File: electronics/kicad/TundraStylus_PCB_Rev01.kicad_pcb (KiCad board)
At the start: 2 copper layers, 80 x 16 mm, 11 parts, among them J1 CON_TPAD, J2 CON_MENU, J3 CON_TRIG, J4 CON_GRIP, SW1 TPAD, SW2 MENU, SW3 TRIG, SW4 GRIP

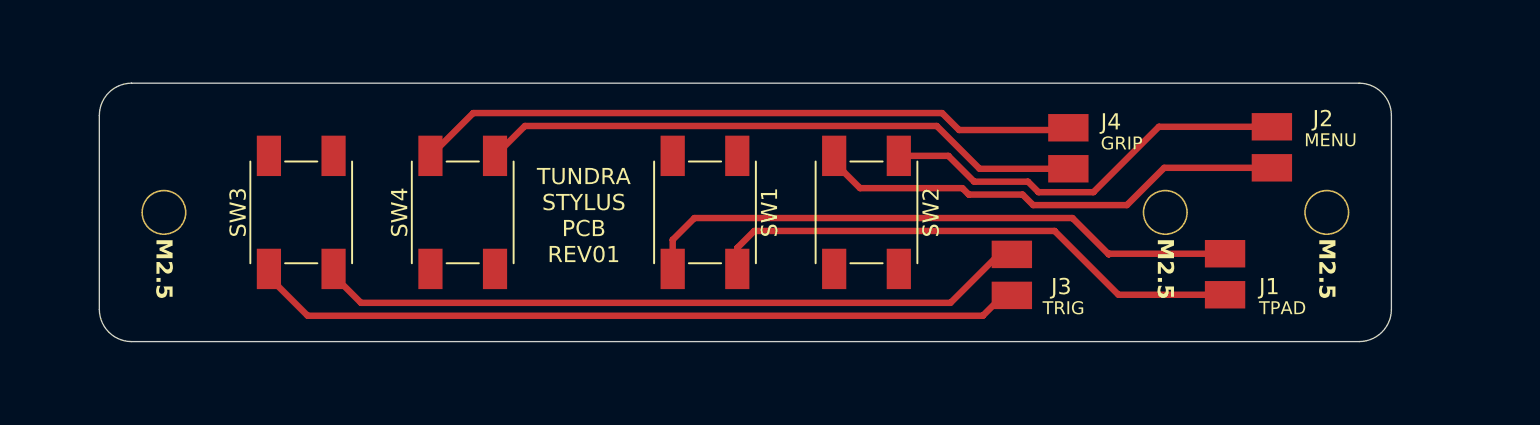
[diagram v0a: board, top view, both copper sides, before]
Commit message: Add latest electronics design
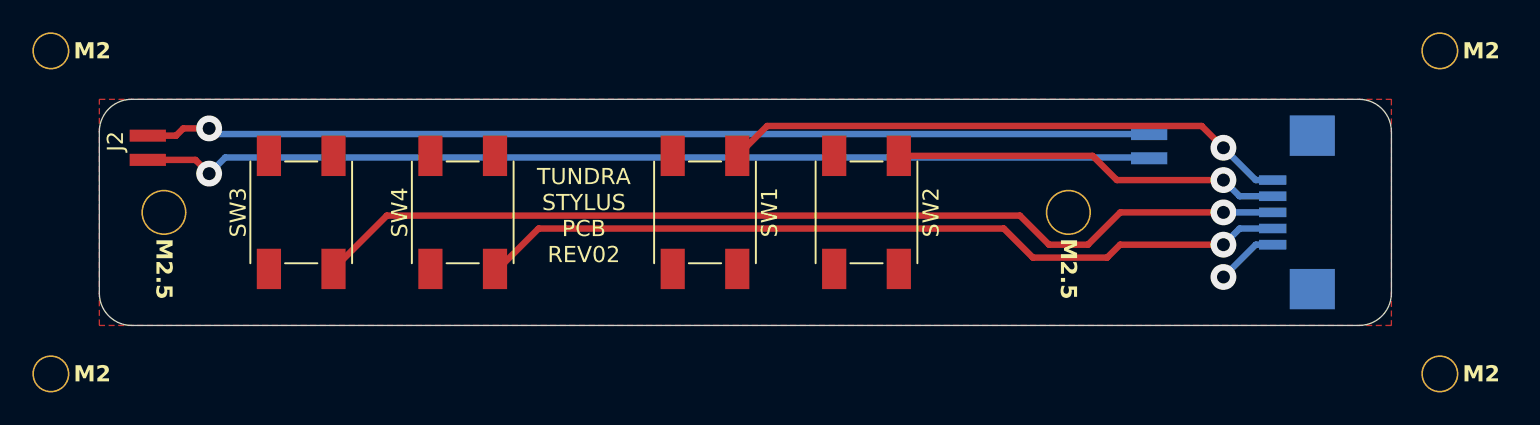
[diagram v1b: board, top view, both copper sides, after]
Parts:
- removed J3: CON_TRIG, fab:PinHeader_1x02_P2.54mm_Horizontal_SMD
- removed J4: CON_GRIP, fab:PinHeader_1x02_P2.54mm_Horizontal_SMD
- added H4: ~, fab:MountingHole_M2, F.Cu at (92.0, 108.0)
- added H5: ~, fab:MountingHole_M2, F.Cu at (178.0, 88.0)
- added H6: ~, fab:MountingHole_M2, F.Cu at (178.0, 108.0)
- added P1: IO, TundraIO:Conn_FFC_1x05_P1mm_SideEntry_GCT_FFC3B11-05-T, B.Cu at (168.7, 98.0)
- H2: footprint fab:MountingHole_M2.5 -> fab:MountingHole_M2
- J1: value CON_TPAD -> HAPT; footprint fab:PinHeader_1x02_P2.54mm_Horizontal_SMD -> TundraIO:Conn_2pos_Plain; moved to B.Cu
- J2: value CON_MENU -> HAPT; footprint fab:PinHeader_1x02_P2.54mm_Horizontal_SMD -> TundraIO:Conn_2pos_Plain
- moved H2 79.6 mm to (92.0, 88.0), turned to 0 degrees
- moved J2 69.6 mm to (98.0, 94.0), turned to 90 degrees
- moved J1 10.3 mm to (160.0, 93.9), turned to 90 degrees
- moved H1 6.00 mm to (155.0, 98.0)
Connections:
- J1 pad 1: TPAD_A -> HAPT_P
- J1 pad 2: TPAD_B -> HAPT_N
- J2 pad 1: MENU_A -> HAPT_P
- J2 pad 2: MENU_B -> HAPT_N
- SW1 pad 1: TPAD_A -> TPAD
- SW1 pad 2: TPAD_B -> PWR_GND
- SW2 pad 1: MENU_A -> MENU
- SW2 pad 2: MENU_B -> PWR_GND
- SW3 pad 1: TRIG_A -> TRIG
- SW3 pad 2: TRIG_B -> PWR_GND
- SW4 pad 1: GRIP_A -> GRIP
- SW4 pad 2: GRIP_B -> PWR_GND
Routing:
- net HAPT_P: track 0.00 -> 62.8 mm, vias 0 -> 1
- net HAPT_N: track 0.00 -> 62.3 mm, vias 0 -> 1
- net TRIG: track 0.00 -> 61.1 mm, vias 0 -> 1
- net GRIP: track 0.00 -> 50.7 mm, vias 0 -> 1
- net TRIG_B: track 48.0 -> 0.00 mm
- net TRIG_A: track 44.3 -> 0.00 mm
- net GRIP_B: track 41.1 -> 0.00 mm
- net TPAD_B: track 37.5 -> 0.00 mm
- net GRIP_A: track 37.4 -> 0.00 mm
- net TPAD: track 0.00 -> 35.3 mm, vias 0 -> 1
- net TPAD_A: track 33.6 -> 0.00 mm
- net MENU_B: track 29.6 -> 0.00 mm
- net MENU_A: track 25.7 -> 0.00 mm
- net MENU: track 0.00 -> 24.2 mm, vias 0 -> 1
- net PWR_GND: track 0.00 -> 3.88 mm, vias 0 -> 1
- added copper zone on F.Cu, net PWR_GND
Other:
- board size 80 x 16 mm -> 80 x 14 mm
- board text added: "TUNDRA STYLUS PCB REV02"
- board text removed: "GRIP"
- board text removed: "MENU"
- board text removed: "TPAD"
- board text removed: "TRIG"
- board text removed: "TUNDRA STYLUS PCB REV01"
